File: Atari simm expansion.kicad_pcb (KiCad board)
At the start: 2 copper layers, 113.2 x 55.8 mm, 30 parts, among them J1 4464_A, J10 PB0..7, J11 RAS_sel, J2 4464_B, J3 4464_A, J4 4464_B, J5 SMMU_A, J6 SMMU_B, J7 MMU_A, J8 MMU_A, J9 Mem_On_Off, U1 SIMM_exp_GAL, U11 DRAM_1MB_4bit, U12 DRAM_1MB_4bit, U13 74LS04, U2 74LS175, U3 74LS157, U4 MMU

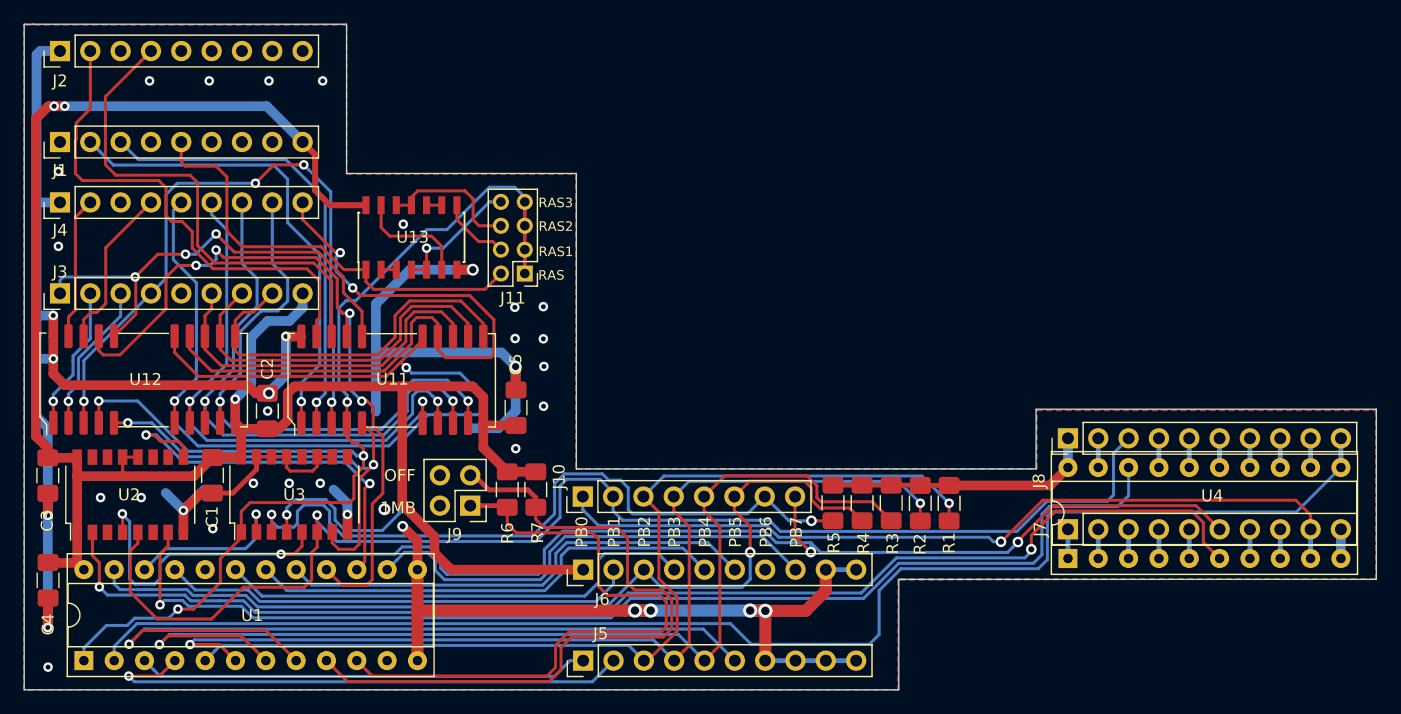
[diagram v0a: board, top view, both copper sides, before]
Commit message: Gerber files
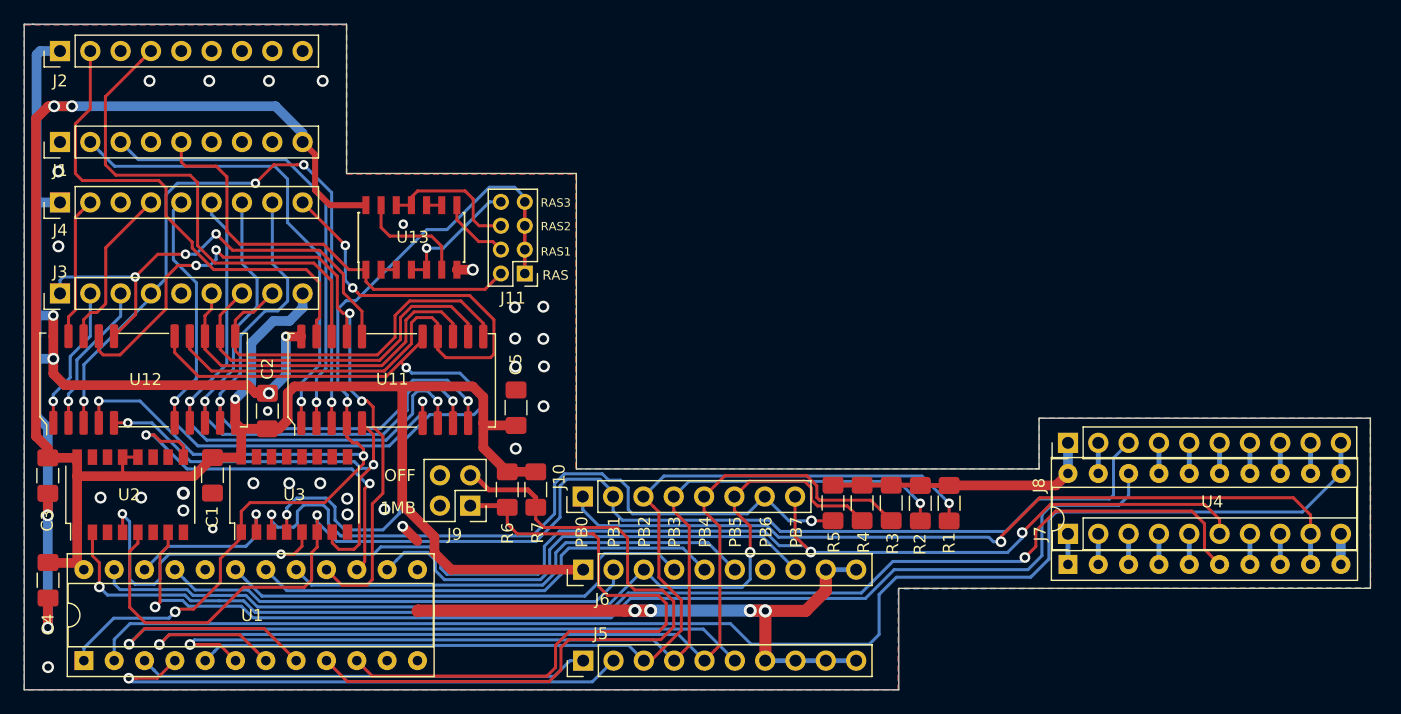
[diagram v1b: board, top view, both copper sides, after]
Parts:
- moved U4 0.50 mm to (190.4, 116.0)
- moved J7 0.38 mm to (190.4, 113.4)
- moved J8 0.38 mm to (190.4, 105.8)
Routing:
- net GND: track 224.3 -> 146.5 mm, vias 38 -> 40
- net RAS_OUT: track 101.9 -> 100.8 mm
- net PB0: track 68.8 -> 69.7 mm
- net VCC: track 176.0 -> 176.7 mm
- net PB1: track 109.3 -> 110.0 mm
- net DQ3: track 41.9 -> 41.3 mm
- net PB7: track 117.1 -> 117.6 mm
- net MAP: track 106.4 -> 106.9 mm
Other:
- board size 113.2 x 55.8 mm -> 112.8 x 55.8 mm
